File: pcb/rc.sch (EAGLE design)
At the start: 67 parts, among them IC2 TP4056

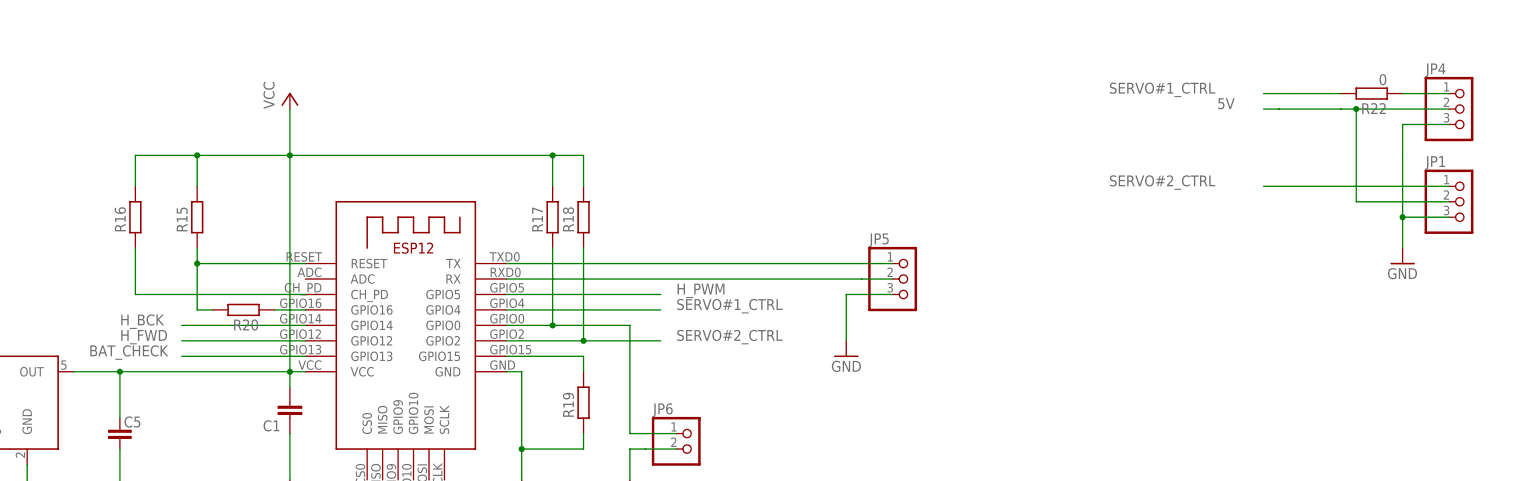
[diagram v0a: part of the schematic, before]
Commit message: pcb
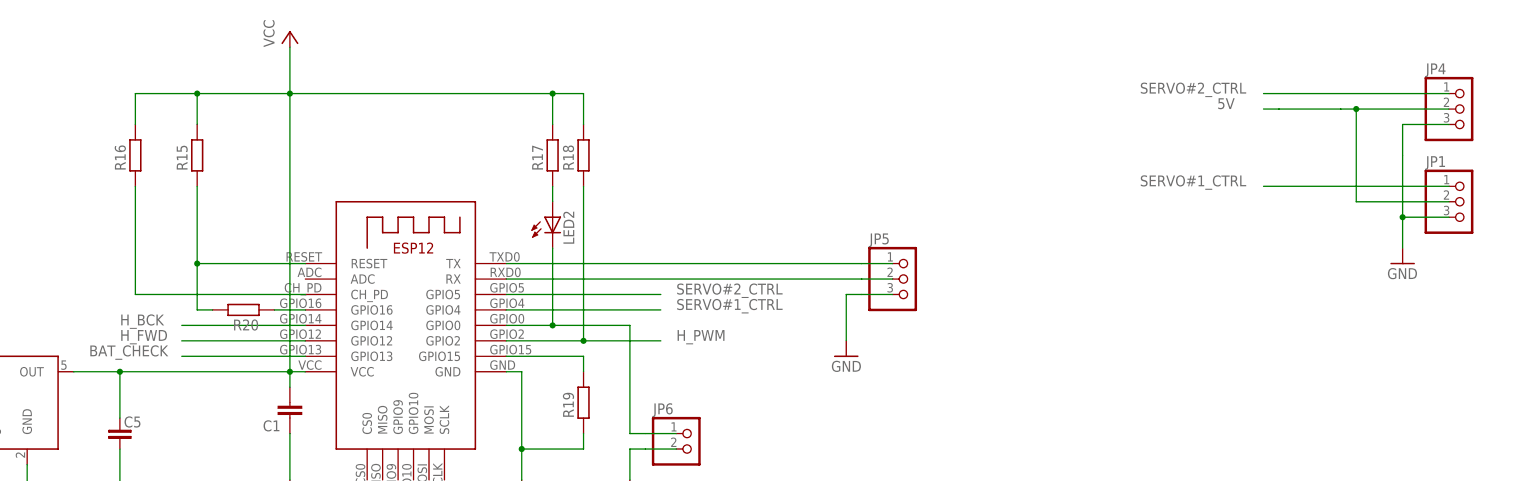
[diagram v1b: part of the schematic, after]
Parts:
- removed R22: 0, skydrop:R_1206
- added LED2: (no value), led:LEDCHIPLED_0805
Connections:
- removed net N$22: JP4.1, R22.1
- new net N$24: LED2.A, R17.1
- net H_PWM: now also R18.1, U1.GPIO2; no longer U1.GPIO5
- net N$21: now also LED2.C; no longer R17.1
- net SERVO#1_CTRL: now also JP1.1; no longer R22.2
- net SERVO#2_CTRL: now also JP4.1, U1.GPIO5; no longer JP1.1, R18.1, U1.GPIO2
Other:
- moved on the sheet: R15, R16, R17, R18
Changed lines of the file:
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@@
 <part name="JP1" library="my" deviceset="PINHD-1X3" device=""/>
 <part name="GND25" library="supply1" library_urn="urn:adsk.eagle:library:371" deviceset="GND" device=""/>
-<part name="R22" library="skydrop" deviceset="R_" device="1206" value="0"/>
 <part name="D1" library="semicon-smd-ipc" library_urn="urn:adsk.eagle:library:353" deviceset="D-FILL-" device="SMB" package3d_urn="urn:adsk.eagle:package:26311/1"/>
+<part name="LED2" library="led" library_urn="urn:adsk.eagle:library:259" deviceset="LED" device="CHIPLED_0805" package3d_urn="urn:adsk.eagle:package:15821/2"/>
 </parts>
 <sheets>
@@
 <instance part="GND5" gate="1" x="241.3" y="33.02"/>
 <instance part="U1" gate="G$1" x="78.74" y="134.62"/>
-<instance part="R15" gate="G$1" x="43.18" y="147.32" rot="R90"/>
-<instance part="R16" gate="G$1" x="33.02" y="147.32" rot="R90"/>
-<instance part="R17" gate="G$1" x="101.6" y="147.32" rot="R90"/>
-<instance part="R18" gate="G$1" x="106.68" y="147.32" rot="R90"/>
-<instance part="P+3" gate="VCC" x="58.42" y="167.64"/>
+<instance part="R15" gate="G$1" x="43.18" y="157.48" rot="R90"/>
+<instance part="R16" gate="G$1" x="33.02" y="157.48" rot="R90"/>
+<instance part="R17" gate="G$1" x="101.6" y="157.48" rot="R90"/>
+<instance part="R18" gate="G$1" x="106.68" y="157.48" rot="R90"/>
+<instance part="P+3" gate="VCC" x="58.42" y="177.8"/>
 <instance part="GND7" gate="1" x="96.52" y="101.6"/>
 <instance part="R19" gate="G$1" x="106.68" y="116.84" rot="R90"/>
@@
 <instance part="JP1" gate="A" x="251.46" y="149.86"/>
 <instance part="GND25" gate="1" x="241.3" y="139.7"/>
-<instance part="R22" gate="G$1" x="236.22" y="167.64" rot="R180"/>
 <instance part="D1" gate="G$1" x="-63.5" y="129.54"/>
+<instance part="LED2" gate="G$1" x="101.6" y="147.32"/>
 </instances>
 <busses>
@@
 <wire x1="60.96" y1="121.92" x2="58.42" y2="121.92" width="0.1524" layer="91"/>
 <pinref part="P+3" gate="VCC" pin="VCC"/>
-<wire x1="58.42" y1="121.92" x2="58.42" y2="157.48" width="0.1524" layer="91"/>
+<wire x1="58.42" y1="121.92" x2="58.42" y2="167.64" width="0.1524" layer="91"/>
 <pinref part="R15" gate="G$1" pin="2"/>
-<wire x1="58.42" y1="157.48" x2="58.42" y2="165.1" width="0.1524" layer="91"/>
-<wire x1="43.18" y1="152.4" x2="43.18" y2="157.48" width="0.1524" layer="91"/>
-<wire x1="43.18" y1="157.48" x2="58.42" y2="157.48" width="0.1524" layer="91"/>
+<wire x1="58.42" y1="167.64" x2="58.42" y2="175.26" width="0.1524" layer="91"/>
+<wire x1="43.18" y1="162.56" x2="43.18" y2="167.64" width="0.1524" layer="91"/>
+<wire x1="43.18" y1="167.64" x2="58.42" y2="167.64" width="0.1524" layer="91"/>
 <pinref part="R17" gate="G$1" pin="2"/>
-<wire x1="58.42" y1="157.48" x2="101.6" y2="157.48" width="0.1524" layer="91"/>
-<wire x1="101.6" y1="157.48" x2="101.6" y2="152.4" width="0.1524" layer="91"/>
+<wire x1="58.42" y1="167.64" x2="101.6" y2="167.64" width="0.1524" layer="91"/>
+<wire x1="101.6" y1="167.64" x2="101.6" y2="162.56" width="0.1524" layer="91"/>
 <pinref part="R18" gate="G$1" pin="2"/>
-<wire x1="106.68" y1="152.4" x2="106.68" y2="157.48" width="0.1524" layer="91"/>
-<wire x1="106.68" y1="157.48" x2="101.6" y2="157.48" width="0.1524" layer="91"/>
-<junction x="101.6" y="157.48"/>
+<wire x1="106.68" y1="162.56" x2="106.68" y2="167.64" width="0.1524" layer="91"/>
+<wire x1="106.68" y1="167.64" x2="101.6" y2="167.64" width="0.1524" layer="91"/>
+<junction x="101.6" y="167.64"/>
 <pinref part="R16" gate="G$1" pin="2"/>
-<wire x1="33.02" y1="152.4" x2="33.02" y2="157.48" width="0.1524" layer="91"/>
-<wire x1="33.02" y1="157.48" x2="43.18" y2="157.48" width="0.1524" layer="91"/>
-<junction x="43.18" y="157.48"/>
-<junction x="58.42" y="157.48"/>
+<wire x1="33.02" y1="162.56" x2="33.02" y2="167.64" width="0.1524" layer="91"/>
+<wire x1="33.02" y1="167.64" x2="43.18" y2="167.64" width="0.1524" layer="91"/>
+<junction x="43.18" y="167.64"/>
+<junction x="58.42" y="167.64"/>
 <pinref part="C1" gate="G$1" pin="2"/>
 <wire x1="58.42" y1="119.38" x2="58.42" y2="121.92" width="0.1524" layer="91"/>
@@
 <pinref part="R15" gate="G$1" pin="1"/>
 <wire x1="60.96" y1="139.7" x2="43.18" y2="139.7" width="0.1524" layer="91"/>
-<wire x1="43.18" y1="139.7" x2="43.18" y2="142.24" width="0.1524" layer="91"/>
+<wire x1="43.18" y1="139.7" x2="43.18" y2="152.4" width="0.1524" layer="91"/>
 <pinref part="R20" gate="G$1" pin="2"/>
 <wire x1="45.72" y1="132.08" x2="43.18" y2="132.08" width="0.1524" layer="91"/>
@@
 <pinref part="R16" gate="G$1" pin="1"/>
 <wire x1="60.96" y1="134.62" x2="33.02" y2="134.62" width="0.1524" layer="91"/>
-<wire x1="33.02" y1="134.62" x2="33.02" y2="142.24" width="0.1524" layer="91"/>
+<wire x1="33.02" y1="134.62" x2="33.02" y2="152.4" width="0.1524" layer="91"/>
 </segment>
 </net>
 <net name="N$21" class="0">
 <segment>
-<pinref part="R17" gate="G$1" pin="1"/>
-<wire x1="101.6" y1="142.24" x2="101.6" y2="129.54" width="0.1524" layer="91"/>
 <pinref part="U1" gate="G$1" pin="GPIO0"/>
 <wire x1="101.6" y1="129.54" x2="93.98" y2="129.54" width="0.1524" layer="91"/>
-<junction x="101.6" y="129.54"/>
 <pinref part="JP6" gate="G$1" pin="1"/>
 <wire x1="121.92" y1="111.76" x2="116.84" y2="111.76" width="0.1524" layer="91"/>
@@
 <wire x1="114.3" y1="129.54" x2="114.3" y2="111.76" width="0.1524" layer="91"/>
 <wire x1="114.3" y1="111.76" x2="116.84" y2="111.76" width="0.1524" layer="91"/>
+<pinref part="LED2" gate="G$1" pin="C"/>
+<wire x1="101.6" y1="142.24" x2="101.6" y2="129.54" width="0.1524" layer="91"/>
+<junction x="101.6" y="129.54"/>
 </segment>
 </net>
 <net name="SERVO#2_CTRL" class="0">
 <segment>
-<pinref part="U1" gate="G$1" pin="GPIO2"/>
-<wire x1="93.98" y1="127" x2="106.68" y2="127" width="0.1524" layer="91"/>
-<pinref part="R18" gate="G$1" pin="1"/>
-<wire x1="106.68" y1="127" x2="106.68" y2="142.24" width="0.1524" layer="91"/>
-<wire x1="106.68" y1="127" x2="119.38" y2="127" width="0.1524" layer="91"/>
-<junction x="106.68" y="127"/>
-<label x="121.92" y="127" size="1.778" layer="95"/>
-</segment>
-<segment>
-<pinref part="JP1" gate="A" pin="1"/>
-<wire x1="248.92" y1="152.4" x2="218.44" y2="152.4" width="0.1524" layer="91"/>
-<label x="193.04" y="152.4" size="1.778" layer="95"/>
+<pinref part="U1" gate="G$1" pin="GPIO5"/>
+<wire x1="93.98" y1="134.62" x2="119.38" y2="134.62" width="0.1524" layer="91"/>
+<label x="121.92" y="134.62" size="1.778" layer="95"/>
+</segment>
+<segment>
+<pinref part="JP4" gate="A" pin="1"/>
+<wire x1="248.92" y1="167.64" x2="218.44" y2="167.64" width="0.1524" layer="91"/>
+<label x="198.12" y="167.64" size="1.778" layer="95"/>
 </segment>
 </net>
@@
 <net name="H_PWM" class="0">
 <segment>
-<pinref part="U1" gate="G$1" pin="GPIO5"/>
-<wire x1="93.98" y1="134.62" x2="119.38" y2="134.62" width="0.1524" layer="91"/>
-<label x="121.92" y="134.62" size="1.778" layer="95"/>
-</segment>
-<segment>
 <pinref part="R5" gate="G$1" pin="2"/>
 <wire x1="-48.26" y1="-27.94" x2="-55.88" y2="-27.94" width="0.1524" layer="91"/>
 <label x="-60.96" y="-22.86" size="1.778" layer="95"/>
+</segment>
+<segment>
+<pinref part="R18" gate="G$1" pin="1"/>
+<pinref part="U1" gate="G$1" pin="GPIO2"/>
+<wire x1="106.68" y1="152.4" x2="106.68" y2="127" width="0.1524" layer="91"/>
+<wire x1="106.68" y1="127" x2="93.98" y2="127" width="0.1524" layer="91"/>
+<wire x1="106.68" y1="127" x2="119.38" y2="127" width="0.1524" layer="91"/>
+<junction x="106.68" y="127"/>
+<label x="121.92" y="127" size="1.778" layer="95"/>
 </segment>
 </net>
@@
 </segment>
 <segment>
-<wire x1="223.52" y1="167.64" x2="218.44" y2="167.64" width="0.1524" layer="91"/>
-<label x="193.04" y="167.64" size="1.778" layer="95"/>
-<pinref part="R22" gate="G$1" pin="2"/>
-<wire x1="231.14" y1="167.64" x2="223.52" y2="167.64" width="0.1524" layer="91"/>
-</segment>
-</net>
-<net name="N$22" class="0">
-<segment>
-<pinref part="JP4" gate="A" pin="1"/>
-<wire x1="243.84" y1="167.64" x2="248.92" y2="167.64" width="0.1524" layer="91"/>
-<pinref part="R22" gate="G$1" pin="1"/>
-<wire x1="241.3" y1="167.64" x2="243.84" y2="167.64" width="0.1524" layer="91"/>
+<pinref part="JP1" gate="A" pin="1"/>
+<wire x1="248.92" y1="152.4" x2="218.44" y2="152.4" width="0.1524" layer="91"/>
+<label x="198.12" y="152.4" size="1.778" layer="95"/>
 </segment>
 </net>
@@
 </segment>
 </net>
+<net name="N$24" class="0">
+<segment>
+<pinref part="R17" gate="G$1" pin="1"/>
+<pinref part="LED2" gate="G$1" pin="A"/>
+<wire x1="101.6" y1="152.4" x2="101.6" y2="149.86" width="0.1524" layer="91"/>
+</segment>
+</net>
